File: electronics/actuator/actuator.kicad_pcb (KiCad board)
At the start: 2 copper layers, 26 parts, among them J1 Screw_Terminal_01x03, Q1 NTMFS4935NT1G, Q2 NTMFS4935NT1G, Q3 NTMFS4935NT1G, Q4 NTMFS4935NT1G, Q5 NTMFS4935NT1G, Q6 NTMFS4935NT1G, U1 drv8323rs

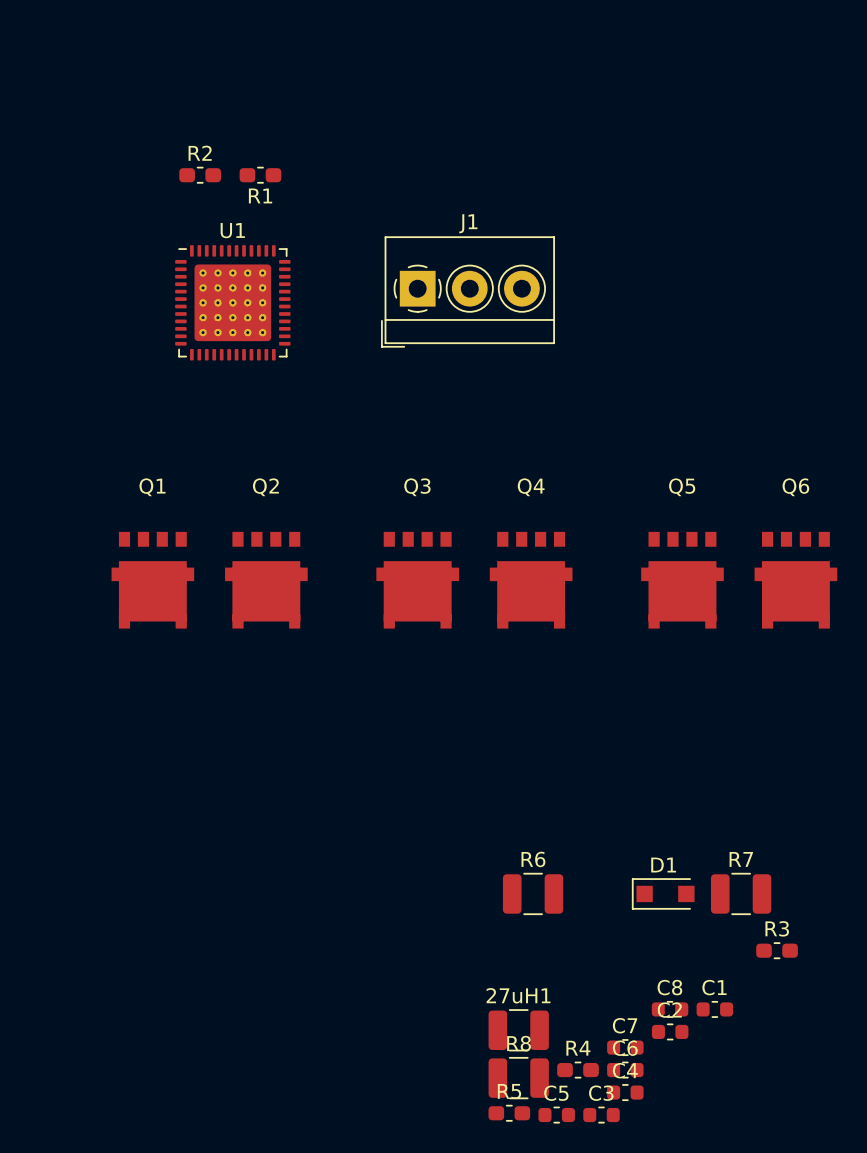
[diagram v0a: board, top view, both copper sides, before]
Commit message: Added a bunch of stuff and initial layout.
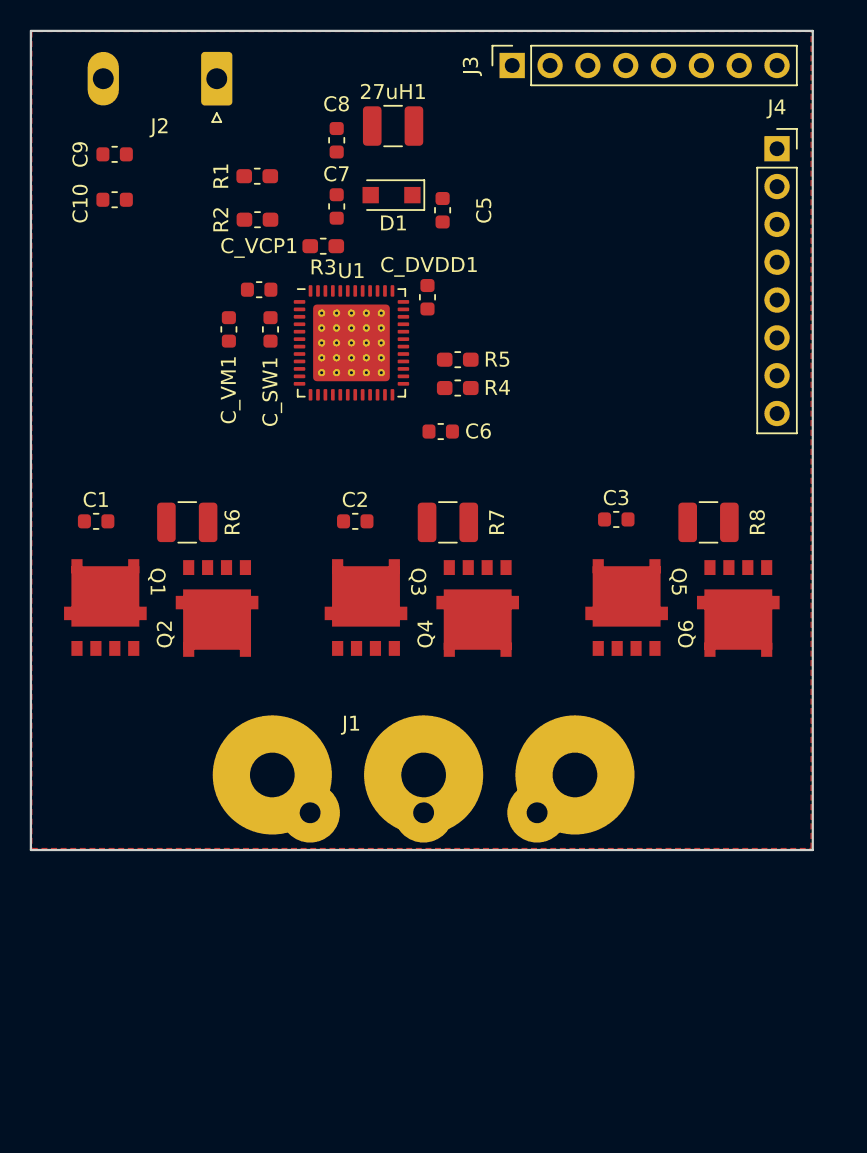
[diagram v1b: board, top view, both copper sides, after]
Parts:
- removed C4: 1uF, Capacitor_SMD:C_0603_1608Metric
- added C10: 10uF, Capacitor_SMD:C_0603_1608Metric, F.Cu at (120.6, 61.3)
- added C9: 10uF, Capacitor_SMD:C_0603_1608Metric, F.Cu at (120.6, 58.3)
- added C_DVDD1: 1uF, Capacitor_SMD:C_0603_1608Metric, F.Cu at (141.6, 67.9)
- added C_SW1: 1uF, Capacitor_SMD:C_0603_1608Metric, F.Cu at (131.1, 70.0)
- added C_VCP1: 47uF, Capacitor_SMD:C_0603_1608Metric, F.Cu at (130.3, 67.4)
- added C_VM1: 0.1uF, Capacitor_SMD:C_0603_1608Metric, F.Cu at (128.3, 70.0)
- added J2: PWR_IN, connectors:PhoenixContact_GMSTBA_2,5_2-G-7,62_1x02_P7.62mm_Horizontal, F.Cu at (127.5, 53.2)
- added J3: Pinouts, Connector_PinSocket_2.54mm:PinSocket_1x08_P2.54mm_Vertical, F.Cu at (147.3, 52.3)
- added J4: Pinouts, Connector_PinSocket_2.54mm:PinSocket_1x08_P2.54mm_Vertical, F.Cu at (165.1, 57.9)
- C1: value 0.1uF -> 10uF
- C2: value 47uF -> 10uF
- C3: value 1uF -> 10uF
- J1: value Screw_Terminal_01x03 -> MOTOR_OUT; footprint TerminalBlock_4Ucon:TerminalBlock_4Ucon_1x03_P3.50mm_Horizontal -> connectors:PhoenixContact_GMSTBA_2,5_3-G-7,62_1x03_P7.62mm_Horizontal
- moved C8 62.5 mm to (135.5, 57.3), turned to 270 degrees
- moved 27uH1 61.3 mm to (139.3, 56.4)
- moved C5 61.2 mm to (142.6, 62.0), turned to 90 degrees
- moved C7 59.7 mm to (135.5, 61.8), turned to 90 degrees
- moved R3 56.3 mm to (134.6, 64.5), turned to 180 degrees
- moved C1 52.9 mm to (119.4, 82.9)
- moved R5 50.7 mm to (143.7, 72.1), turned to 180 degrees
- moved D1 50.4 mm to (139.2, 61.0), turned to 180 degrees
- moved R4 46.5 mm to (143.7, 74.0), turned to 180 degrees
- moved C6 44.6 mm to (142.5, 76.9), turned to 180 degrees
- moved C2 40.3 mm to (136.8, 82.9)
- moved C3 40.0 mm to (154.3, 82.8)
- moved R8 39.4 mm to (160.5, 83.0), turned to 180 degrees
- moved J1 35.9 mm to (133.8, 102.5)
- moved R6 34.1 mm to (125.5, 83.0), turned to 180 degrees
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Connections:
- 27uH1 pad 1: VCC -> VAA
- C2 pad 1: Net-(C2-Pad1) -> VDRAIN
- C2 pad 2: Net-(C2-Pad2) -> SNA
- C3 pad 1: Net-(C3-Pad1) -> VDRAIN
- C3 pad 2: VDRAIN -> SNA
- C7 pad 1: VDRAIN -> VCC
- C8 pad 1: VCC -> VAA
- R1 pad 1: VCC -> VAA
- R3 pad 1: VDRAIN -> VCC
- R4 pad 1: VCC -> VAA
- R5 pad 1: VCC -> VAA
- U1 pad 3: Net-(C2-Pad1) -> Net-(C_VCP1-Pad1)
- U1 pad 4: Net-(C2-Pad2) -> Net-(C_VCP1-Pad2)
- U1 pad 47: VDRAIN -> VCC
- U1 pad 5: Net-(C3-Pad1) -> Net-(C_SW1-Pad1)
- U1 pad 6: VDRAIN -> VCC
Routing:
- added copper zone on F.Cu, net SNA
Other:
- board outline added: 52.5 x 55 mm
